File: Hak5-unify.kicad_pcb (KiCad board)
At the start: 2 copper layers, 26 x 17.5 mm, 4 parts, among them J1 Conn_01x04, J2 Conn_01x03, U1 Unify-Nano

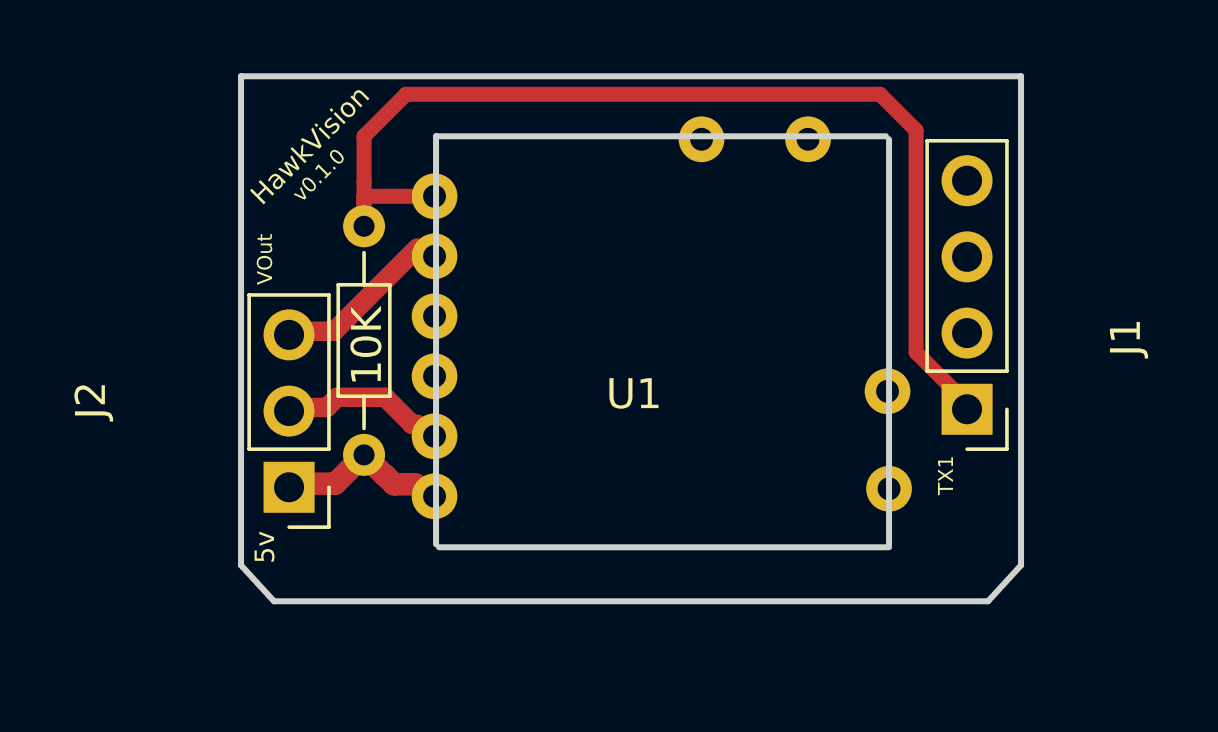
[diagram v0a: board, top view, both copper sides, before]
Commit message: v0.1.1
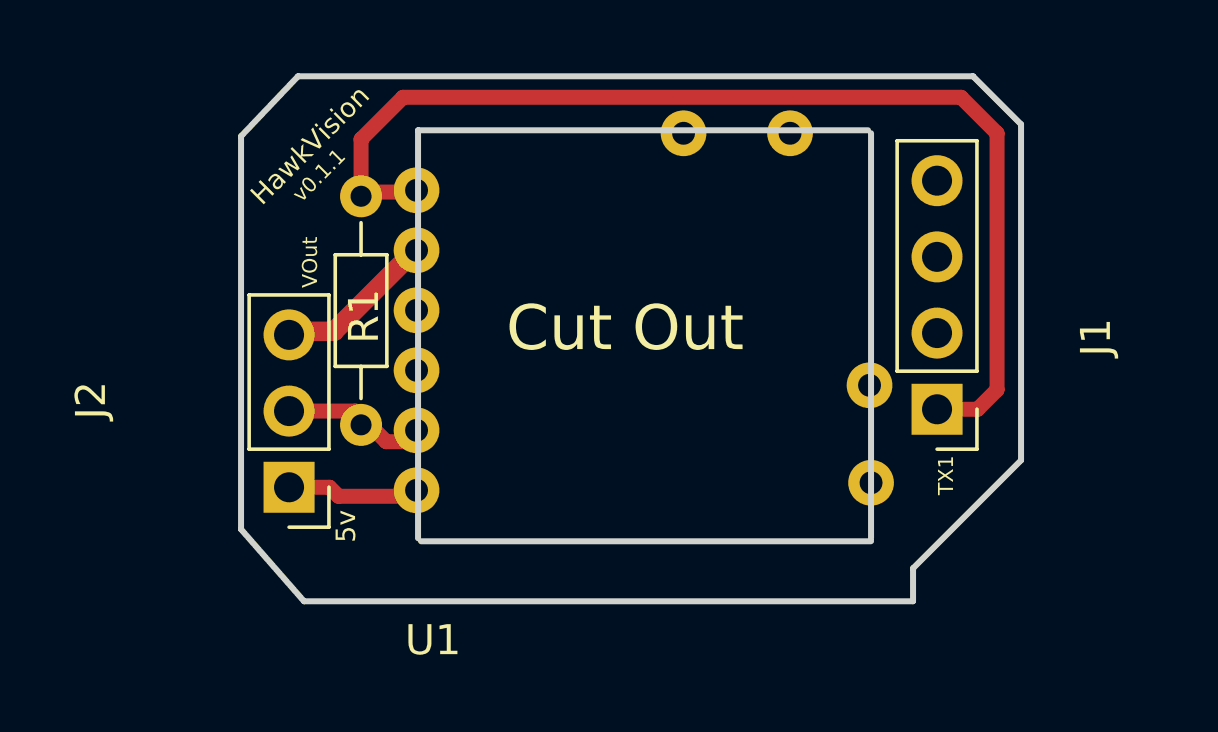
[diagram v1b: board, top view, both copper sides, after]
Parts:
- removed 10K: R, Resistors_ThroughHole:R_Axial_DIN0204_L3.6mm_D1.6mm_P7.62mm_Horizontal
- added R1: R, Resistors_ThroughHole:R_Axial_DIN0204_L3.6mm_D1.6mm_P7.62mm_Horizontal, F.Cu at (104.0, 86.5)
- moved J1 1.00 mm to (123.2, 93.6)
- moved U1 0.63 mm to (106.1, 97.8)
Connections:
- J2 pad 1: Net-(J2-Pad1) -> +5V
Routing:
- net TX: track 35.3 -> 36.8 mm
- net +5V: track 5.03 -> 4.47 mm
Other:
- outline, holes or cut-outs redrawn
- board text added: "Cut Out"
- board text added: "v0.1.1"
- board text removed: "v0.1.0"
